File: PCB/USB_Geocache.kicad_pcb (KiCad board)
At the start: 4 copper layers, 40 x 40 mm, 60 parts, among them J1 USB_B_Mini, J2 USB_ALT, P2 Battery, P3 SWD, P4 GPS, P5 Button, P7 Servo, Q1 DMP3099L, Q2 DMP3099L, Q3 DMP3099L, Q4 DMP3099L, U1 MCP73831-2-OT, U2 LM3670MF, U3 STM32F072C8Tx, U4 CR2013-MI2120, U5 25LC640A-I/SN, Y1 8MHz

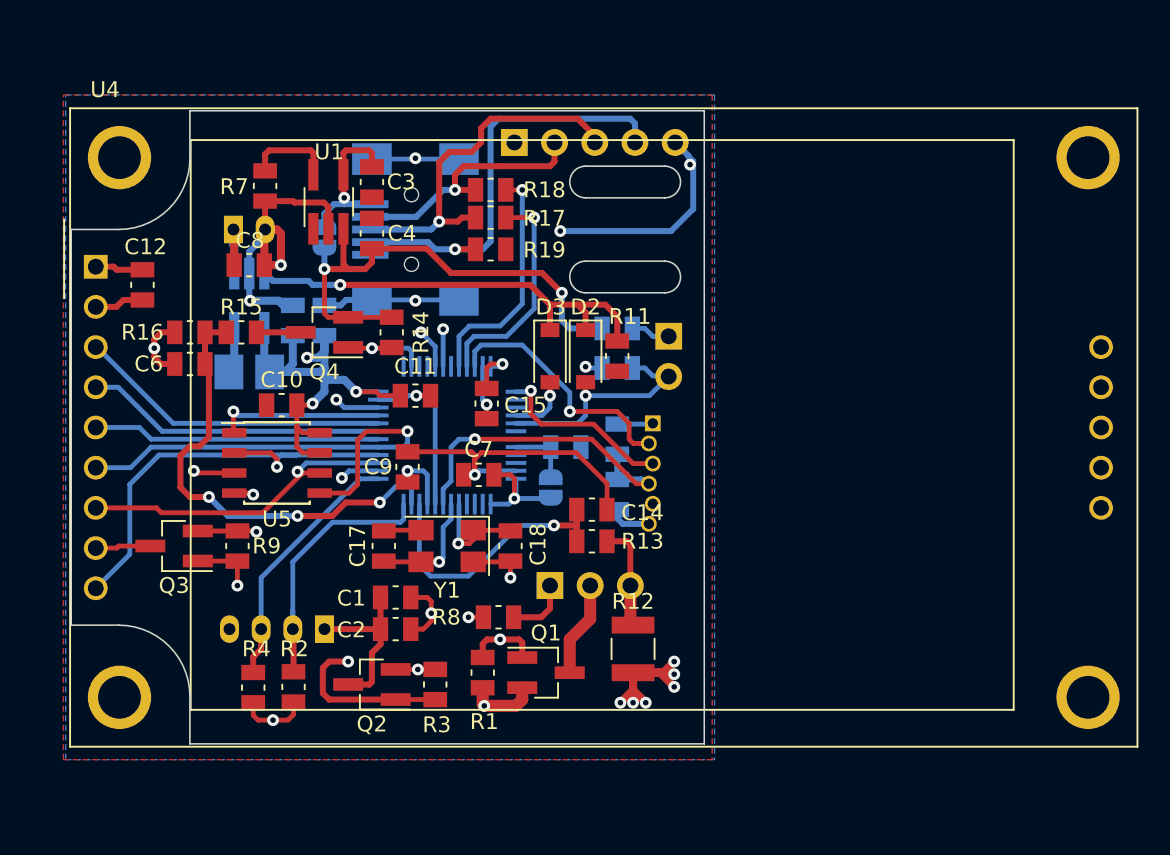
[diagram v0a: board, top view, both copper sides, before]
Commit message: PCB / BOM stuff
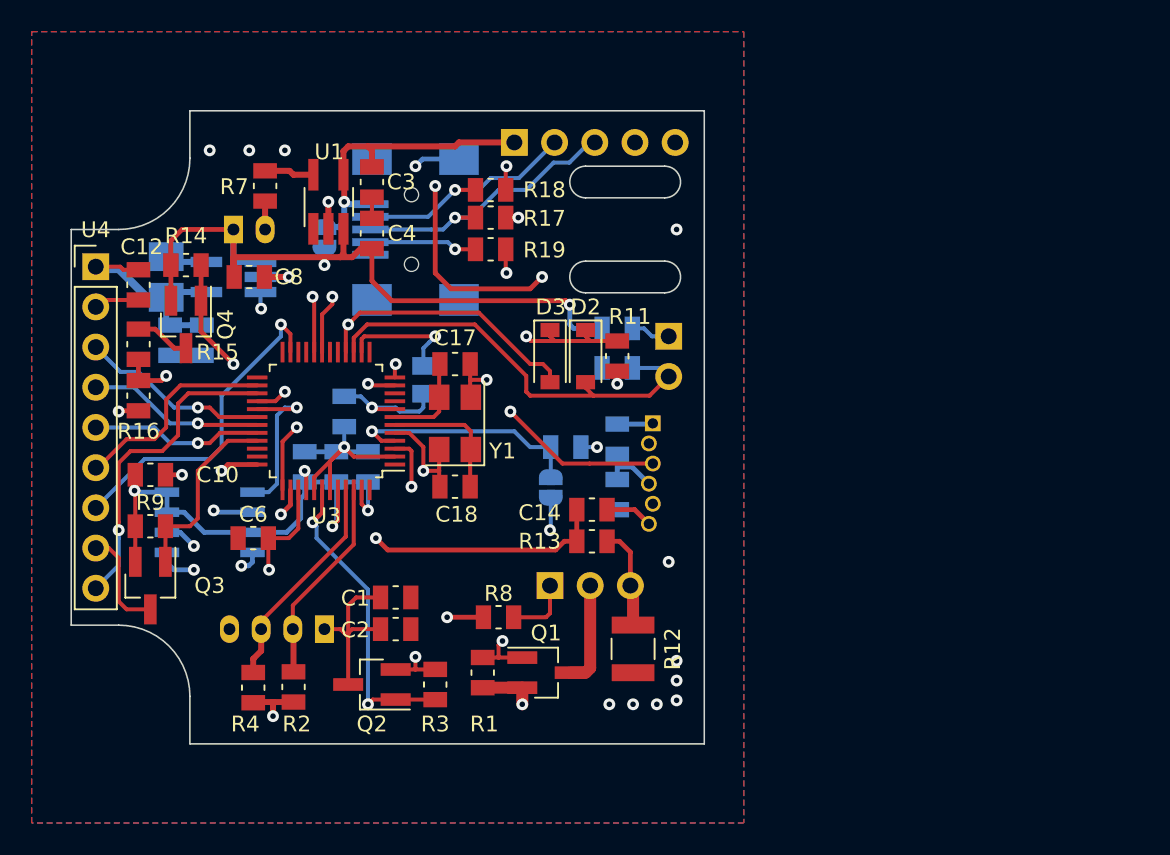
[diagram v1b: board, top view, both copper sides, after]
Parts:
- added R21: 10K, Resistor_SMD:R_0805_2012Metric, B.Cu at (199.8, 77.0)
- C11, C15, C7, C9: value C -> 0.1uF; moved to B.Cu
- C6: value C -> 10uF
- R17, R18: value R -> 0
- R19: value R -> 100K
- U3: value STM32F072C8Tx -> LPC11U68JBD48E; footprint Package_QFP:TQFP-48_7x7mm_P0.5mm -> Package_QFP:LQFP-48_7x7mm_P0.5mm; moved to F.Cu
- U4: footprint Display:CR2013-MI2120 -> Connector_PinHeader_2.54mm:PinHeader_1x09_P2.54mm_Vertical
- U5: moved to B.Cu
- moved R14 13.7 mm to (184.8, 69.8), turned to 0 degrees
- moved C17 12.3 mm to (201.8, 76.0), turned to 0 degrees
- moved C6 11.7 mm to (189.0, 87.0)
- moved C15 10.3 mm to (194.2, 82.5), turned to 90 degrees
- moved C10 9.39 mm to (182.5, 83.0), turned to 180 degrees
- moved Q4 8.76 mm to (184.8, 73.5), turned to 270 degrees
- moved L1 7.97 mm to (183.5, 70.5), turned to 90 degrees
- moved C13 7.85 mm to (183.8, 74.5), turned to 270 degrees
- moved C16 7.85 mm to (185.8, 74.5), turned to 270 degrees
- moved Y1 7.77 mm to (201.8, 79.8), turned to 90 degrees
- moved U3 7.70 mm to (193.6, 79.6), turned to 180 degrees
- moved C7 7.02 mm to (196.2, 82.5), turned to 90 degrees
- moved R15 6.54 mm to (181.8, 74.8), turned to 270 degrees
- moved C9 6.50 mm to (192.2, 82.5)
- moved U5 5.67 mm to (186.2, 86.0), turned to 180 degrees
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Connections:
- C17 pad 1: Net-(C17-Pad1) -> /OSC2
- C18 pad 1: Net-(C18-Pad1) -> /OSC1
- P3 pad 5: Net-(P3-Pad5) -> (no net)
- Q3 pad 3: Net-(Q3-Pad3) -> (no net)
- U1 pad 1: Net-(U1-Pad1) -> (no net)
- U3 pad 1: +3V3 -> (no net)
- U3 pad 10: /I_SERVO -> (no net)
- U3 pad 11: /V_BATT -> /SERVO_EN
- U3 pad 12: /GPS_TX -> /SERVO_PWM
- U3 pad 13: /GPS_RX -> (no net)
- U3 pad 14: /GPS_PWR -> Net-(R21-Pad2)
- U3 pad 15: /SPI_SCK -> /BUTTON
- U3 pad 16: /SPI_MISO -> /SW_ENABLE
- U3 pad 17: /SPI_MOSI -> (no net)
- U3 pad 18: /LCD_DC -> (no net)
- U3 pad 19: /LCD_RESET -> /USB_D-
- U3 pad 2: Net-(U3-Pad2) -> GND
- U3 pad 20: /LCD_CS -> /USB_D+
- U3 pad 21: /CS_EEPROM -> (no net)
- U3 pad 22: /LDC_BL -> (no net)
- U3 pad 23: GND -> /SPI_SCK
- U3 pad 24: +3V3 -> (no net)
- U3 pad 25: Net-(U3-Pad25) -> (no net)
- U3 pad 26: /VMEAS_CTRL -> /SPI_MOSI
- U3 pad 27: Net-(U3-Pad27) -> /SPI_MISO
- U3 pad 28: Net-(U3-Pad28) -> /SWCLK
- U3 pad 29: /SERVO_PWM -> /CS_EEPROM
- U3 pad 3: Net-(U3-Pad3) -> /SW_RESET
- U3 pad 30: /SERVO_EN -> (no net)
- U3 pad 31: Net-(U3-Pad31) -> (no net)
- U3 pad 32: /USB_D- -> (no net)
- U3 pad 33: /USB_D+ -> /LDC_BL
- U3 pad 34: /SWDIO -> (no net)
- U3 pad 35: GND -> (no net)
- U3 pad 36: +3V3 -> /VMEAS_CTRL
- U3 pad 37: /SWCLK -> /SWDIO
- U3 pad 38: Net-(U3-Pad38) -> /I_SERVO
- U3 pad 39: Net-(U3-Pad39) -> /V_BATT
- U3 pad 4: Net-(U3-Pad4) -> Net-(JP1-Pad2)
- U3 pad 40: /SW_ENABLE -> +3V3
- U3 pad 41: /BUTTON -> GND
- U3 pad 42: Net-(U3-Pad42) -> /GPS_PWR
- U3 pad 43: Net-(U3-Pad43) -> GND
- U3 pad 44: Net-(JP1-Pad2) -> +3V3
- U3 pad 45: Net-(U3-Pad45) -> /GPS_RX
- U3 pad 46: Net-(U3-Pad46) -> /GPS_TX
- U3 pad 47: GND -> +3V3
- U3 pad 48: +3V3 -> (no net)
- U3 pad 5: Net-(C18-Pad1) -> GND
- U3 pad 6: Net-(C17-Pad1) -> /OSC1
- U3 pad 7: /SW_RESET -> /OSC2
- U3 pad 8: GND -> +3V3
- U3 pad 9: +3V3 -> (no net)
- Y1 pad 1: Net-(C18-Pad1) -> /OSC1
- Y1 pad 3: Net-(C17-Pad1) -> /OSC2
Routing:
- net GND: track 124.3 -> 69.1 mm, vias 20 -> 23
- net (no net): track 0.00 -> 40.8 mm, vias 0 -> 3
- net +3V3: track 63.9 -> 84.9 mm
- net /SWDIO: track 16.0 -> 36.7 mm
- net /SWCLK: track 11.4 -> 31.5 mm, vias 1 -> 2
- net /LCD_CS: track 19.8 -> 0.00 mm
- net /LCD_RESET: track 19.0 -> 0.00 mm
- net /LCD_DC: track 18.2 -> 0.00 mm
- net /SW_ENABLE: track 3.96 -> 17.1 mm
- net /BUTTON: track 15.0 -> 27.7 mm, vias 1 -> 0
- net +BATT: track 106.0 -> 93.8 mm
- net Net-(JP1-Pad2): track 4.10 -> 15.6 mm, vias 0 -> 1
- net /LDC_BL: track 23.0 -> 12.0 mm, vias 2 -> 0
- net /VMEAS_CTRL: track 6.33 -> 16.6 mm, vias 1 -> 2
- net /SPI_SCK: track 21.0 -> 30.1 mm, vias 1 -> 2
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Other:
- board text added: "Reverse Geocache Rev C Sept. 2018"
- board text removed: "Reverse Geocache Rev C March 2018"
